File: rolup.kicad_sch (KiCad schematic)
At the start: 10 parts, among them J1 switch, J2 phto, J3 bala paiin, J4 k a, J5 k b, J6 Conn_01x10_Pin, J7 k b

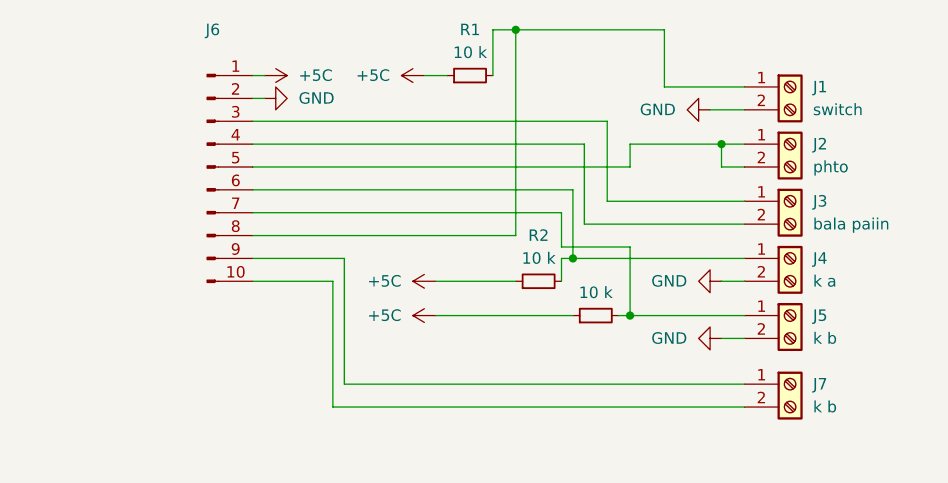
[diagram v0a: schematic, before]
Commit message: pcb
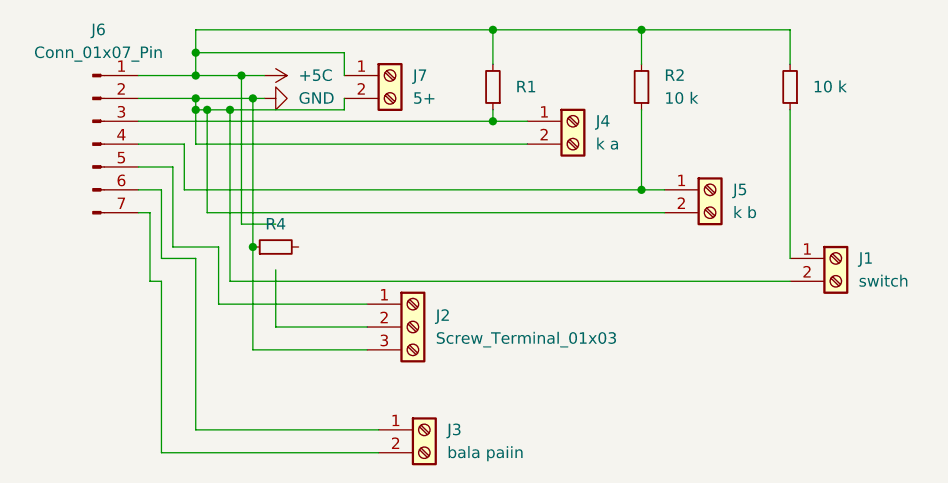
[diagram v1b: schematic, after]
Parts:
- removed J2: phto, symbol Connector:Screw_Terminal_01x02
- removed J6: Conn_01x10_Pin, Connector_Wuerth:Wuerth_WR-WTB_64801011622_1x10_P1.50mm_Vertical, symbol Connector:Conn_01x10_Pin
- added J2: Screw_Terminal_01x03, TerminalBlock_MetzConnect:TerminalBlock_MetzConnect_Type011_RT05503HBWC_1x03_P5.00mm_Horizontal, symbol Connector:Screw_Terminal_01x03
- added J6: Conn_01x07_Pin, Connector_TE-Connectivity:TE_826576-7_1x07_P3.96mm_Vertical, symbol Connector:Conn_01x07_Pin
- added R4: 10 k, Resistor_THT:R_Axial_DIN0204_L3.6mm_D1.6mm_P7.62mm_Horizontal, symbol Device:R_Small
- J1: footprint TerminalBlock:TerminalBlock_bornier-2_P5.08mm -> TerminalBlock_MetzConnect:TerminalBlock_MetzConnect_Type011_RT05502HBWC_1x02_P5.00mm_Horizontal
- J3, J4, J5: footprint (none) -> TerminalBlock_MetzConnect:TerminalBlock_MetzConnect_Type011_RT05502HBWC_1x02_P5.00mm_Horizontal
- J7: value k b -> 5+; footprint (none) -> TerminalBlock_MetzConnect:TerminalBlock_MetzConnect_Type011_RT05502HBWC_1x02_P5.00mm_Horizontal
- R1, R2, R3: footprint (none) -> Resistor_THT:R_Axial_DIN0204_L3.6mm_D1.6mm_P7.62mm_Horizontal
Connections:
- net +5C: now also J7.1 (Pin_1), R1.2, R2.2, R3.2, J6.1 (Pin_1); no longer R1.1, R2.1, R3.1
- net GND: now also J7.2 (Pin_2), J2.3 (Pin_3), J6.2 (Pin_2), R4.1
- net at J1.1 (Pin_1): now also R3.1; no longer R1.2
- net at J5.1 (Pin_1): now also R2.1, J6.4 (Pin_4); no longer R3.2
- net at J3.1 (Pin_1): now also J6.6 (Pin_6)
- net at J3.2 (Pin_2): now also J6.7 (Pin_7)
- net at J4.1 (Pin_1): now also R1.1, J6.3 (Pin_3); no longer R2.2
- new net: J2.1 (Pin_1), J6.5 (Pin_5)
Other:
- moved on the sheet: J1, J3, J4, J5, J7, R1, R2
